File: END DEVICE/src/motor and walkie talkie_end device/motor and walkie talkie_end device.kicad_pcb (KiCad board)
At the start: 2 copper layers, 77.9 x 49.7 mm, 118 parts, among them IC1 LM4871MX, IC2 BQ24616RGER, IC4 TPS55340RTER, J1 ICSP, J2 FTDI_CONN, J3 speaker_conn, J4 Barrel_Jack_Switch, J5 Motor_Out, J6 BATT_CONN, Q1 DMP6185SE, Q2 DMP6185SE, Q3 IRF540NPBF, Q4 IRF540NPBF, Q5 IRF540NPBF, Q6 DMP6185SE, SW3 SW_Push, SW6 SW_SPDT, U1 ATmega328P-MU, U2 Ai-Thinker-Ra-02, U3 SA818-1W, U4 LP_Filter, U5 MCP41010, U6 LM1117-3.3(, U9 L4931ABDT50, Y1 16MHz

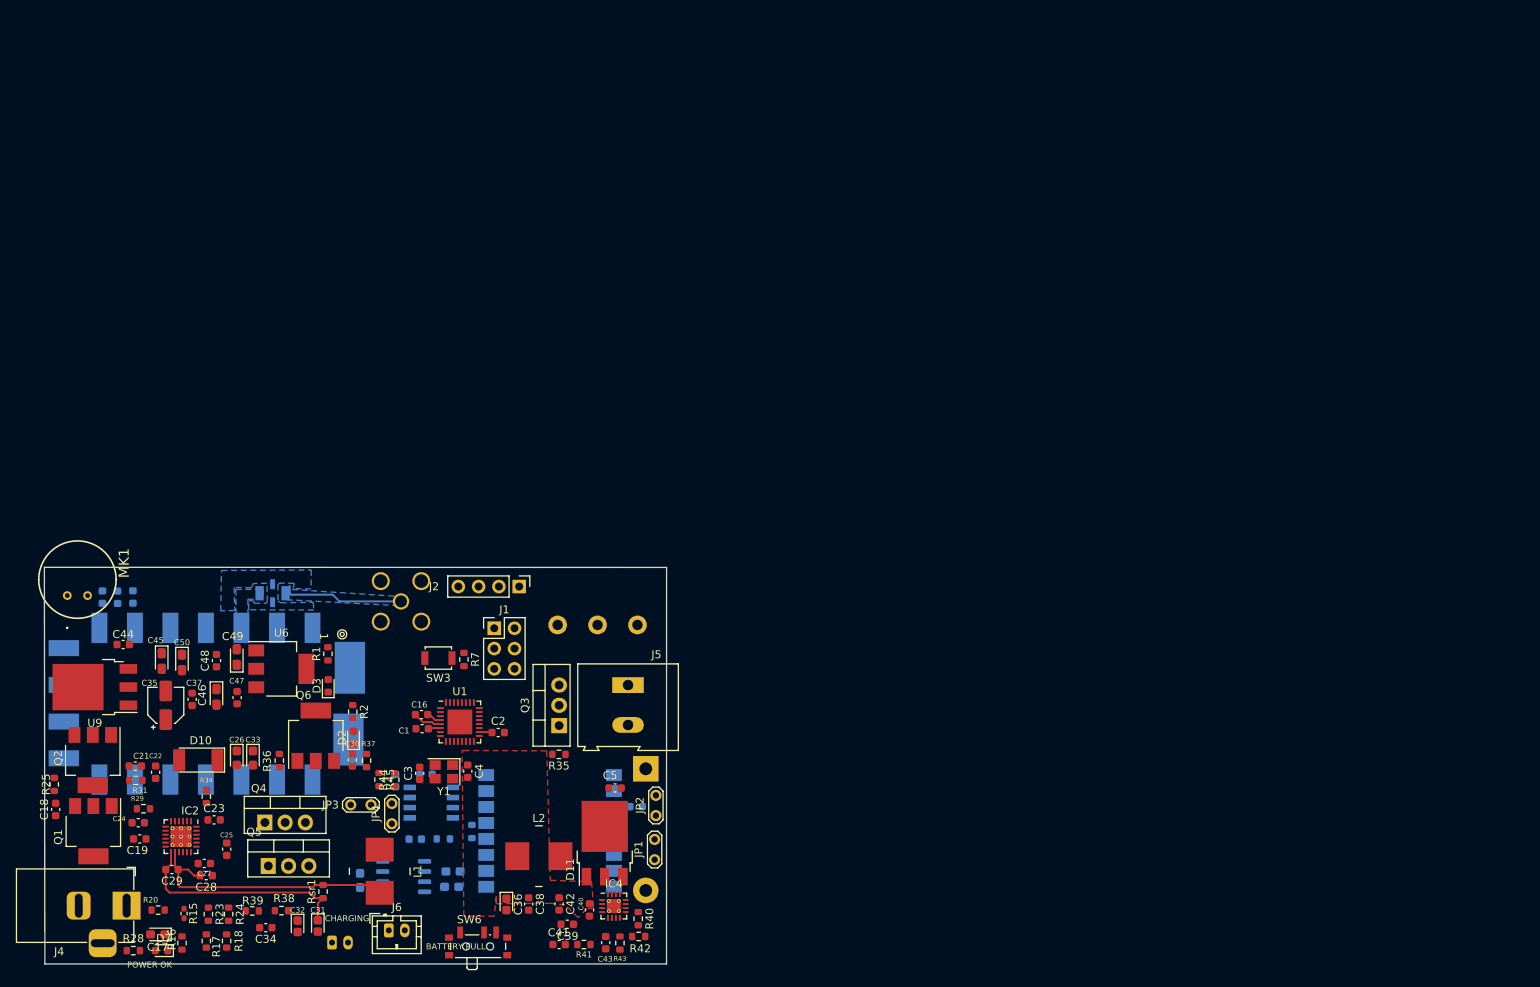
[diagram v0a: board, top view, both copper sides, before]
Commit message: 90% complete and. PCB done with tracks and design rules verified as well as dimensions
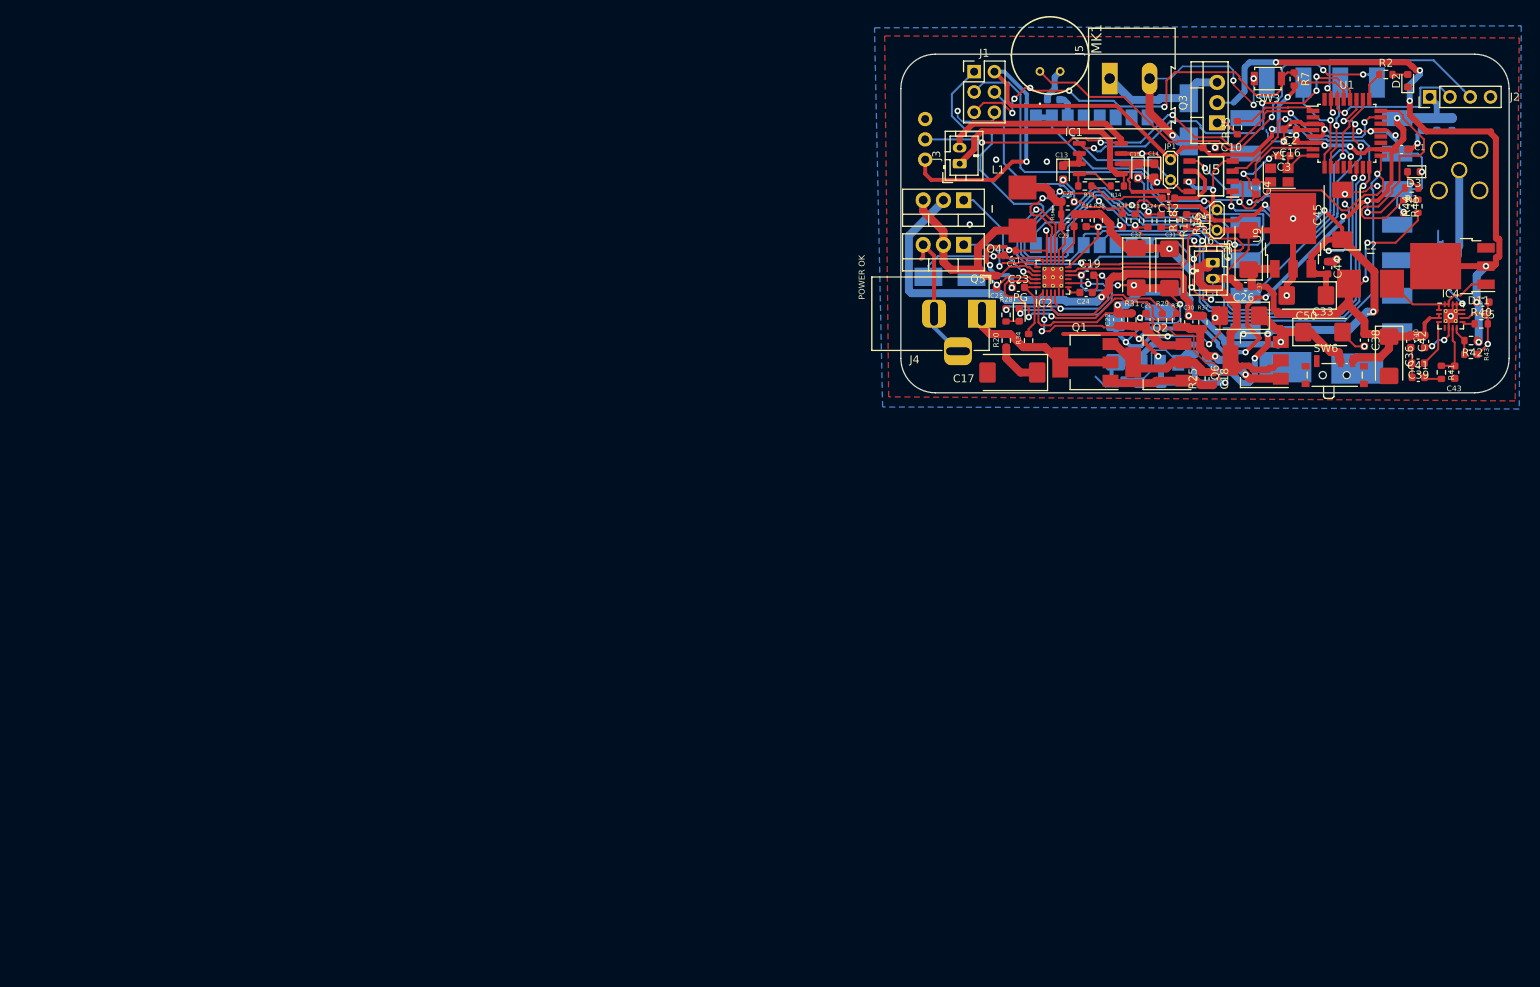
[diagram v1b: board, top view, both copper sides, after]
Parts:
- removed C11: 10nF, Capacitor_SMD:C_0603_1608Metric
- removed D10: 1N6858UR, Diode_SMD:D_MELF
- removed JP3, JP4: Jumper, TestPoint:TestPoint_2Pads_Pitch2.54mm_Drill0.8mm
- added D4: B320B-13-F, Diode_SMD:D_SMB_Handsoldering, B.Cu at (125.4, 111.4)
- C10, C12, C13, IC1, J3, R13, R14, U5: moved to F.Cu
- C14: value 1.0uF -> 1.0uF_TCMIA106AT; moved to F.Cu
- C15: value 10nF -> 1.0uF_TCMIA106AT; moved to F.Cu
- C17: value 2.2uF -> 2.2uF_TCKIX225DT; footprint Capacitor_Tantalum_SMD:CP_EIA-2012-12_Kemet-R -> Capacitor_Tantalum_SMD:CP_EIA-7343-31_Kemet-D
- C26, C33: footprint Capacitor_Tantalum_SMD:CP_EIA-2012-12_Kemet-R -> Capacitor_Tantalum_SMD:CP_EIA-6032-28_Kemet-C
- C31, C32: footprint Capacitor_Tantalum_SMD:CP_EIA-1608-10_AVX-L -> Capacitor_Tantalum_SMD:CP_EIA-6032-28_Kemet-C
- C35: footprint Capacitor_SMD:CP_Elec_4x4.5 -> Capacitor_Tantalum_SMD:CP_EIA-6032-28_Kemet-C
- C36: value 10uF_50V -> 10uF_>30V; footprint Capacitor_Tantalum_SMD:CP_EIA-1608-08_AVX-J -> Capacitor_Tantalum_SMD:CP_EIA-6032-28_Kemet-C
- C45: footprint Capacitor_Tantalum_SMD:CP_EIA-2012-12_Kemet-R_Pad1.30x1.05mm_HandSolder -> Capacitor_Tantalum_SMD:CP_EIA-7343-31_Kemet-D
- C46: footprint Capacitor_Tantalum_SMD:CP_EIA-2012-12_Kemet-R_Pad1.30x1.05mm_HandSolder -> Capacitor_Tantalum_SMD:CP_EIA-6032-28_Kemet-C; moved to B.Cu
- C47, C48, U6: moved to B.Cu
- C49: footprint Capacitor_Tantalum_SMD:CP_EIA-2012-12_Kemet-R_Pad1.30x1.05mm_HandSolder -> Capacitor_Tantalum_SMD:CP_EIA-3216-18_Kemet-A; moved to B.Cu
- C50: footprint Capacitor_Tantalum_SMD:CP_EIA-2012-12_Kemet-R_Pad1.30x1.05mm_HandSolder -> Capacitor_Tantalum_SMD:CP_EIA-6032-28_Kemet-C
- D1: value 1N5406 -> RS2K-13-F; footprint Diode_THT:D_DO-201AD_P15.24mm_Horizontal -> Diode_SMD:D_SMB_Handsoldering
- RV1: footprint Potentiometer_THT:Potentiometer_Piher_PC-16_Single_Horizontal -> Potentiometer_THT:Potentiometer_Vishay_148-149_Single_Horizontal
- U1: value ATmega328P-MU -> ATmega328-AU; footprint Package_DFN_QFN:QFN-32-1EP_5x5mm_P0.5mm_EP3.1x3.1mm -> Package_QFP:TQFP-32_7x7mm_P0.8mm
- moved C8 179.1 mm to (188.3, 92.3), turned to 270 degrees
- moved C6 175.6 mm to (186.4, 92.3), turned to 270 degrees
- moved C7 172.0 mm to (184.5, 92.3), turned to 270 degrees
- moved U3 171.9 mm to (162.4, 87.1), turned to 270 degrees
- moved U9 160.4 mm to (168.4, 106.2), turned to 90 degrees
- moved C45 158.1 mm to (174.6, 103.6), turned to 90 degrees
- moved C44 158.1 mm to (172.7, 110.3), turned to 90 degrees
- moved D2 155.6 mm to (182.8, 86.9)
- moved R16 155.0 mm to (155.1, 104.4), turned to 90 degrees
- moved C18 154.7 mm to (158.4, 124.2), turned to 270 degrees
- moved R15 153.5 mm to (156.4, 104.8)
- moved R25 152.4 mm to (156.9, 124.2)
- moved U4 152.3 mm to (189.0, 107.1)
- moved R2 152.1 mm to (180.0, 86.1), turned to 0 degrees
- moved R17 151.1 mm to (153.4, 104.4)
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- renumbered D7 to PG
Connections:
- net BATT_VOLT renamed /BATT_VOLTAGE
- net LM_SD renamed /LM_SD
- net MCURX renamed /MCU_RX
- net MCU_TX renamed /MCU_TX
- net MOTOR_DRV renamed /MOTOR_DRV
- net PD renamed /PD
- net PTT renamed /PTT
- net SCK renamed /SCK
- net lora_SS renamed /LORA_SS
- net pot_CS renamed /POT_CS
- C22 pad 1: BATT_IN -> TO_SYS
- C26 pad 1: BATT_IN -> TO_SYS
- C3 pad 1: Net-(C3-Pad1) -> /oscout
- C30 pad 2: BATT_IN -> TO_SYS
- C33 pad 1: BATT_IN -> TO_SYS
- C35 pad 1: BATT_IN -> /power sheet 2/BATT_IN
- C36 pad 1: BATT_IN -> /power sheet 2/BATT_IN
- C37 pad 1: BATT_IN -> /power sheet 2/BATT_IN
- C38 pad 1: BATT_IN -> /power sheet 2/BATT_IN
- C4 pad 1: Net-(C4-Pad1) -> /oscin
- C40 pad 1: BATT_IN -> /power sheet 2/BATT_IN
- C42 pad 1: BATT_IN -> /power sheet 2/BATT_IN
- IC2 pad 1: BATT_IN -> TO_SYS
- IC4 pad 2: BATT_IN -> /power sheet 2/BATT_IN
- IC4 pad 3: BATT_IN -> /power sheet 2/BATT_IN
- J1 pad 1: MISO -> /MISO
- J1 pad 4: MOSI -> /MOSI
- L2 pad 1: BATT_IN -> /power sheet 2/BATT_IN
- Q4 pad 2: BATT_IN -> TO_SYS
- Q6 pad 3: BATT_IN -> TO_SYS
- R31 pad 1: BATT_IN -> TO_SYS
- R37 pad 1: BATT_IN -> TO_SYS
- R44 pad 1: BATT_IN -> /power sheet 2/BATT_IN
- SW6 pad 2: +BATT -> TO_SYS
- SW6 pad 3: BATT_IN -> /power sheet 2/BATT_IN
- U1 pad 15: MOSI -> /MOSI
- U1 pad 16: MISO -> /MISO
- U1 pad 7: Net-(C3-Pad1) -> /oscin
- U1 pad 8: Net-(C4-Pad1) -> /oscout
- U2 pad 13: MISO -> /MISO
- U2 pad 14: MOSI -> /MOSI
- U5 pad 3: MOSI -> /MISO
- U5 pad 4: Net-(JP4-Pad2) -> /COMMUNICATION/Lora_GND
- U5 pad 7: Net-(JP4-Pad2) -> /COMMUNICATION/Lora_GND
- U5 pad 8: Net-(JP3-Pad2) -> /COMMUNICATION/Lora_3.3V
- U9 pad 1: BATT_IN -> /power sheet 2/BATT_IN
- Y1 pad 1: Net-(C4-Pad1) -> /oscin
- Y1 pad 3: Net-(C3-Pad1) -> /oscout
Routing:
- net GND: track 3.63 -> 357.3 mm, vias 0 -> 54
- net +3V3: track 5.04 -> 202.8 mm, vias 0 -> 15
- net /SCK: track 0.00 -> 138.7 mm, vias 0 -> 3
- net /MISO: track 0.00 -> 135.3 mm, vias 0 -> 2
- net +5V: track 0.00 -> 123.1 mm, vias 0 -> 5
- net TO_SYS: track 0.00 -> 115.0 mm, vias 0 -> 4
- net /MOSI: track 0.00 -> 105.1 mm, vias 0 -> 1
- net /COMMUNICATION/Lora_GND: track 0.00 -> 95.0 mm, vias 0 -> 5
- net 18V: track 0.00 -> 83.5 mm, vias 0 -> 6
- net /LORA_SS: track 0.00 -> 70.3 mm, vias 0 -> 1
- net /VOL: track 0.00 -> 66.0 mm, vias 0 -> 5
- net /POWER sheet 1/vref: track 0.00 -> 65.5 mm, vias 0 -> 4
- net /power sheet 2/BATT_IN: track 0.00 -> 65.1 mm, vias 0 -> 2
- net /RESET: track 0.00 -> 59.6 mm, vias 0 -> 5
- net Net-(MK1-Pad1): track 0.00 -> 55.0 mm, vias 0 -> 3
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- added copper zone on F.Cu, net GND
- removed copper zone on F.Cu, net BATT_IN
- removed copper zone on B.Cu, net Net-(AE1-Pad1)
- removed copper zone on B.Cu, net Net-(JP3-Pad2)
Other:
- board size 77.9 x 49.7 mm -> 76.2 x 42.4 mm
- board text removed: "1"
- board text removed: "BATTERY FULL"
- board text removed: "CHARGING"
